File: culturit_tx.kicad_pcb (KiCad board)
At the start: 4 copper layers, 50 x 52 mm, 132 parts, among them J1 USB4105-GF-A, J2 Battery, J3 FTR-105-02-L-D, SW1 PCM12SMTR, SW2 EVQ-P7J01P, SW3 EVQ-P7J01P, U1 MCP73832T-2ACI_MC, U10 TPS22916CNYFPT, U11 SN74AUP2G08RSER, U12 TPS22916CNYFPT, U13 MDBT50Q-1M, U14 BMM150, U15 BHI260AP, U16 DS28E05R+T, U17 W25Q32JWZPIQ, U2 CSD25304W1015, U3 DMN65D8L-7, U4 CSD25304W1015, U5 TPS3839A09DBZR, U6 TPS22916CNYFPT, U7 LP5907QMFX-2.8Q1, U8 TPS6282618DMQR, U9 SN74AUP2G08RSER, Y1 32.768kHz

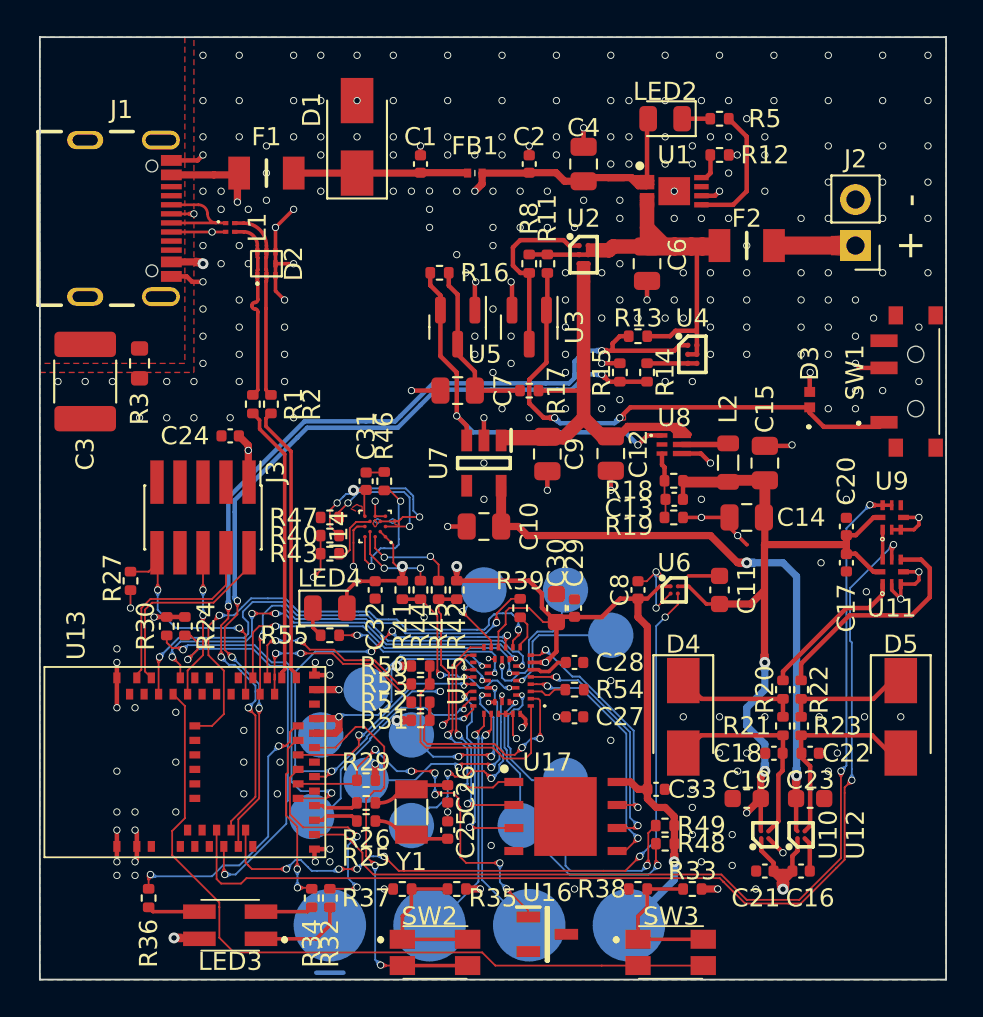
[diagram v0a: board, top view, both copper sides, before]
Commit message: 2022-08-24
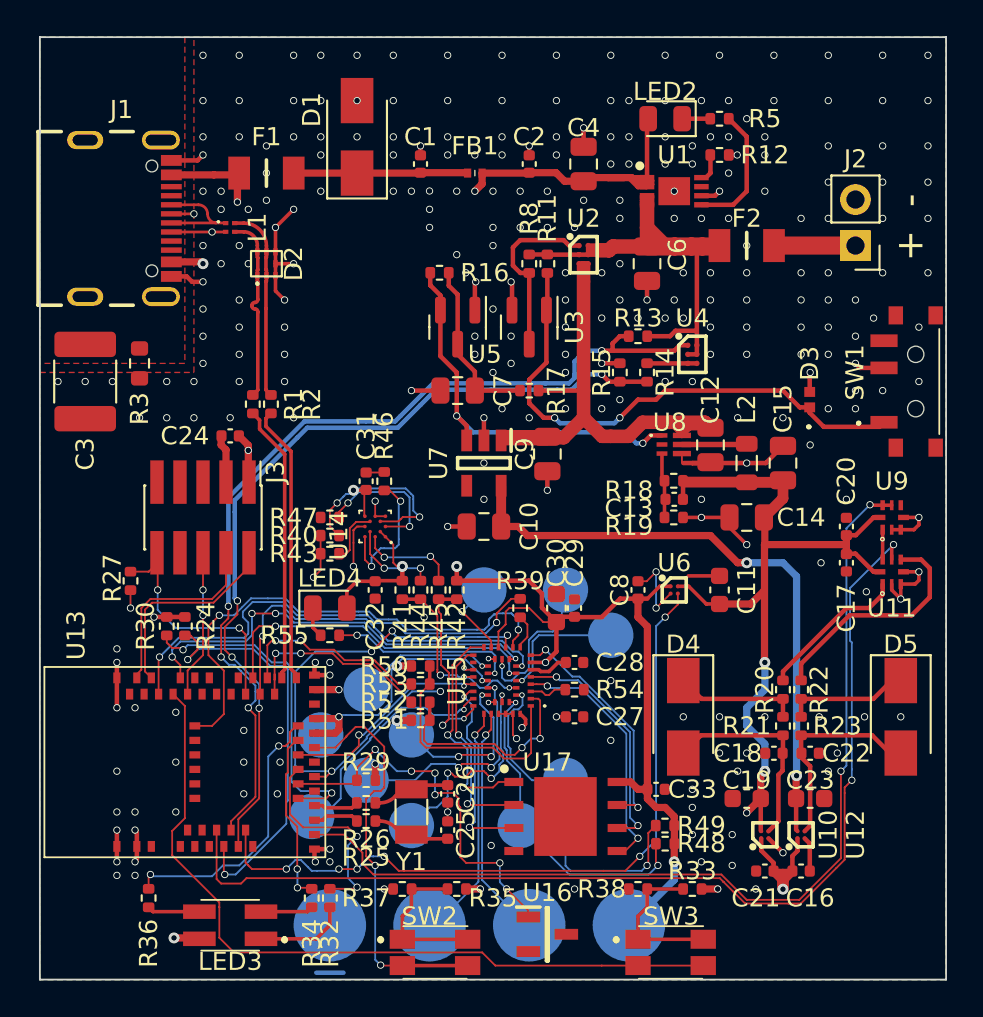
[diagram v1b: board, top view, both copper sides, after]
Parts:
- moved C12 5.52 mm to (57.0, 37.5)
- moved L2 1.03 mm to (59.0, 38.5)
- moved C15 1.00 mm to (61.0, 38.5)
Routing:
- net Earth: track 73.9 -> 79.7 mm, vias 280 -> 281
- net Net-(L2-Pad1): track 7.55 -> 3.10 mm
- net /Power/VDRAIN: track 43.7 -> 41.6 mm
- net +1V8: track 114.2 -> 115.7 mm
- net Net-(D3-Pad1): track 28.7 -> 29.5 mm

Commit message: 2022-09-07
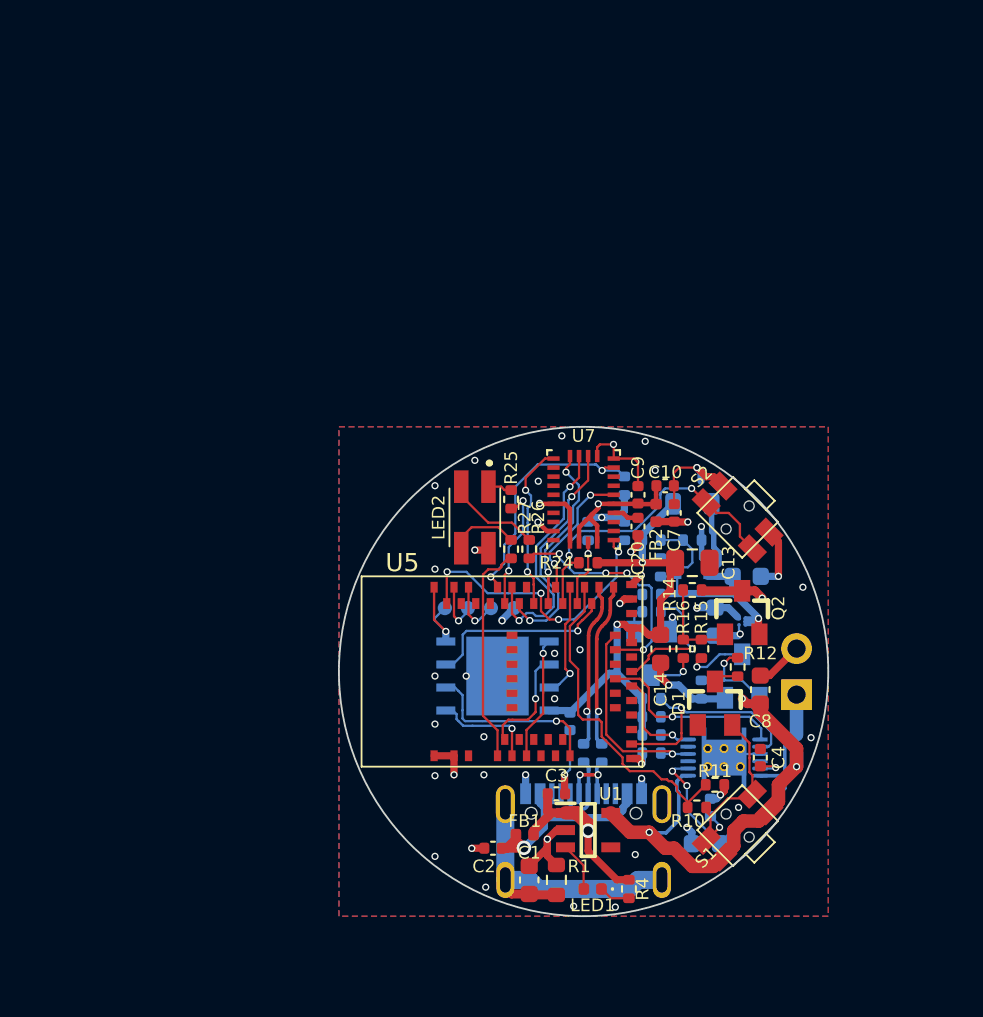
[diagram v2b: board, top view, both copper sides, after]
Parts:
- removed C15: 10uF(2012), Capacitor_SMD:C_0805_2012Metric
- removed C17, C18, C21, C22, C27, C29, C31, C32, C33: 100nF, Capacitor_SMD:C_0402_1005Metric
- removed C19, C23, C30: 1uF(1608), Capacitor_SMD:C_0603_1608Metric
- removed C24: 100pF, Capacitor_SMD:C_0402_1005Metric
- removed C25, C26: 12pF, Capacitor_SMD:C_0402_1005Metric
- removed C28: 200nF, Capacitor_SMD:C_0402_1005Metric
- removed D2: VBUS052CD-FAH-GS08, Local_devices:LLP1713-7L
- removed D3: LXES1UTAA1-157, Local_devices:LXES1UTAA1157
- removed D4, D5: SMAJ7.0A, Diode_SMD:D_SMA
- removed F1: 0ZCJ0050AF2E, Local_devices:FUSC3216X120N
- removed F2: 0ZCJ0075FF2E, Local_devices:FUSC3216X120N
- removed J3: FTR-105-02-L-D, Connector_PinHeader_1.27mm:PinHeader_2x05_P1.27mm_Vertical_SMD
- removed L2: 470nH, Inductor_SMD:L_0805_2012Metric
- removed LED3: IN-P32TATRGB, Local_devices:INP32TATRGB
- removed LED4: ORANGE, LED_SMD:LED_0805_2012Metric
- removed R22, R32: 100, Resistor_SMD:R_0402_1005Metric
- removed R23: 1.91k, Resistor_SMD:R_0402_1005Metric
- removed R33, R35: NC, Resistor_SMD:R_0402_1005Metric
- removed R34, R36: 33, Resistor_SMD:R_0402_1005Metric
- removed R37, R38: 360, Resistor_SMD:R_0402_1005Metric
- removed R39, R40, R43, R44, R45, R46, R47, R52, R53, R54: 0, Resistor_SMD:R_0402_1005Metric
- removed R41, R42, R48, R49, R50, R51: 4.7k, Resistor_SMD:R_0402_1005Metric
- removed R55: 470, Resistor_SMD:R_0402_1005Metric
- removed SW1: PCM12SMTR, Local_devices:PCM12SMTR
- removed SW2, SW3: EVQ-P7J01P, Local_devices:EVQP7J01P
- removed TP1, TP10, TP11, TP12, TP14, TP15, TP2, TP3, TP4, TP5, TP9: TestPoint, TestPoint:TestPoint_Pad_D2.5mm
- removed TP13, TP6, TP7, TP8: TestPoint, TestPoint:TestPoint_Pad_D4.0mm
- removed U10, U12: TPS22916CNYFPT, Local_devices:BGA4C40P2X2_78X78X50
- removed U11, U9: SN74AUP2G08RSER, Local_devices:RSE0008A
- removed U13: MDBT50Q-1M, Local_devices:MDBT50Q-1M
- removed U14: BMM150, Package_CSP:WLCSP-12_1.56x1.56mm_P0.4mm
- removed U15: BHI260AP, Local_devices:BHI260AP
- removed U16: DS28E05R+T, Local_devices:SOT95P237X112-3N
- removed U17: W25Q32JWZPIQ, Local_devices:SON127P600X500X80-9N-D
- removed U8: TPS6282618DMQR, Local_devices:TPS6282618DMQR
- removed Y1: 32.768kHz, Crystal:Crystal_SMD_3215-2Pin_3.2x1.5mm
- added C5: 10uF/1608, Capacitor_SMD:C_0603_1608Metric, B.Cu at (56.8, 59.5)
- added CN1: 2.54 X 2P, Connector_PinHeader_2.54mm:PinHeader_1x02_P2.54mm_Vertical, B.Cu at (61.8, 51.3)
- added FB2: MMZ1005Y121CT000, Inductor_SMD:L_0402_1005Metric, F.Cu at (54.0, 41.2)
- added LED1: APHHS1005SURCK, LED_SMD:LED_0402_1005Metric, F.Cu at (50.5, 62.0)
- added Q1: MMBT2222LT1G, Local_devices:SOT23, B.Cu at (58.8, 50.2)
- added Q2: FDN340P, Local_devices:SOT23, F.Cu at (58.8, 46.8)
- added Q3: MMBT2222LT1G, Local_devices:SOT23, B.Cu at (53.8, 49.0)
- added R10: 10k, Resistor_SMD:R_0402_1005Metric, F.Cu at (56.2, 57.5)
- added R28: 10k, Resistor_SMD:R_0402_1005Metric, B.Cu at (52.2, 39.8)
- added R4: 330, Resistor_SMD:R_0402_1005Metric, F.Cu at (52.5, 62.0)
- added R6: WFCP0402R0100FE66, Resistor_SMD:R_0402_1005Metric, B.Cu at (61.8, 54.0)
- added R7: 10k, Resistor_SMD:R_0402_1005Metric, B.Cu at (53.8, 54.5)
- added R9: 10k, Resistor_SMD:R_0402_1005Metric, B.Cu at (53.8, 51.5)
- added S1: SKSCLDE010, Local_devices:SKSCLDE010, F.Cu at (58.5, 58.5)
- added S2: SKSCLDE010, Local_devices:SKSCLDE010, F.Cu at (58.5, 41.5)
- C1: value 100nF, 16V -> 4.7nF/1608; footprint Capacitor_SMD:C_0402_1005Metric -> Capacitor_SMD:C_0603_1608Metric
- C10, C7: value 2.2uF(2012) -> 10nF; footprint Capacitor_SMD:C_0805_2012Metric -> Capacitor_SMD:C_0402_1005Metric
- C11: value 1uF(1608) -> 4.7uF/1608; moved to B.Cu
- C12: value 4.7uF(2012) -> 1uF(1608); footprint Capacitor_SMD:C_0805_2012Metric -> Capacitor_SMD:C_0603_1608Metric; moved to B.Cu
- C13: value 120pF -> 22uF/2012; footprint Capacitor_SMD:C_0402_1005Metric -> Capacitor_SMD:C_0805_2012Metric
- C14: value 10uF(2012) -> 10uF; footprint Capacitor_SMD:C_0805_2012Metric -> Capacitor_SMD:C_0603_1608Metric
- C16, R2: moved to B.Cu
- C2: value 220nF, 16V -> 10nF
- C3: value 1nF(1812),X7R,2kV -> 100nF; footprint Capacitor_SMD:C_1812_4532Metric -> Capacitor_SMD:C_0402_1005Metric
- C4: value 4.7uF(2012) -> 100nF; footprint Capacitor_SMD:C_0805_2012Metric -> Capacitor_SMD:C_0402_1005Metric
- C6: value 4.7uF(2012) -> 10nF; footprint Capacitor_SMD:C_0805_2012Metric -> Capacitor_SMD:C_0402_1005Metric; moved to B.Cu
- C8: value 100nF -> 1uF(1608); footprint Capacitor_SMD:C_0402_1005Metric -> Capacitor_SMD:C_0603_1608Metric
- C9: value 2.2uF(2012) -> 100nF; footprint Capacitor_SMD:C_0805_2012Metric -> Capacitor_SMD:C_0402_1005Metric
- D1: value SMAJ7.0A -> MMBD4148; footprint Diode_SMD:D_SMA -> Local_devices:SOT23
- FB1: value BLM15AG700SN1D -> MMZ1005Y121CT000; footprint Local_devices:BLM15AG700SN1D -> Inductor_SMD:L_0402_1005Metric
- J1: value USB4105-GF-A -> SWD; footprint Local_devices:GCT_USB4105-GF-A -> Local_devices:SWD_port; moved to B.Cu
- J2: value Battery -> USB4105-GF-A; footprint Connector_PinHeader_2.54mm:PinHeader_1x02_P2.54mm_Vertical -> Local_devices:GCT_USB4105-GF-A; moved to B.Cu
- L1: value DLM0QSN500HY2D -> 1uH/2012; footprint Local_devices:DLM0QSB120HY2D -> Inductor_SMD:L_0805_2012Metric; moved to B.Cu
- LED2: value ORANGE -> IN-P32TATRGB; footprint LED_SMD:LED_0805_2012Metric -> Local_devices:INP32TATRGB
- R1: value 22 -> 1M(1608); footprint Resistor_SMD:R_0402_1005Metric -> Resistor_SMD:R_0603_1608Metric
- R11: value 2M -> 20k
- R13: value 1M -> 20k; moved to B.Cu
- R14: value 300k -> 100k
- R15: value 180k -> 1k
- R16: value 0 -> 1k
- R17: value 1k -> 100k; moved to B.Cu
- R18: value 200k -> 1k; moved to B.Cu
- R19: value 100k -> 499k; moved to B.Cu
- R20: value 100 -> 200k; moved to B.Cu
- R21: value 1.91k -> 100k; moved to B.Cu
- R24: value 4.7k -> 10k
- R25: value 0 -> 100
- R26: value 0 -> 33
- R27: value 10k -> 33
- R29, R30: value 4.7k -> 10k; moved to B.Cu
- R3: value 1M(1608) -> 22; footprint Resistor_SMD:R_0603_1608Metric -> Resistor_SMD:R_0402_1005Metric; moved to B.Cu
- R5: value 470 -> 10k; moved to B.Cu
- R8: value 1M -> 10k; moved to B.Cu
- U1: value MCP73832T-2ACI_MC -> MAX1555EZK+T; footprint Local_devices:SON50P300X200X100-9N-D -> Local_devices:SOT95P275X110-5N
- U2: value CSD25304W1015 -> BQ27441DRZR-G1A; footprint Local_devices:BGA6C50P2X3_95X145X62 -> Local_devices:IC_BQ27441DRZR-G1A; moved to B.Cu
- U3: value DMN65D8L-7 -> TPS62A01ADRLR; footprint Package_TO_SOT_SMD:SOT-23 -> Local_devices:SOTFL50P160X60-6N; moved to B.Cu
- U4: value CSD25304W1015 -> TCR3UG33A,LF; footprint Local_devices:BGA6C50P2X3_95X145X62 -> Local_devices:BGA4N35P2X2_64X64X33; moved to B.Cu
- U5: value TPS3839A09DBZR -> MDBT50Q-1M; footprint Package_TO_SOT_SMD:SOT-23 -> Local_devices:MDBT50Q-1M
- U6: value TPS22916CNYFPT -> W25Q32JWZPIQ; footprint Local_devices:BGA4C40P2X2_78X78X50 -> Local_devices:SON127P600X500X80-9N-D; moved to B.Cu
- U7: value LP5907QMFX-2.8Q1 -> BNO055; footprint Local_devices:SOT95P280X145-5N -> Package_LGA:LGA-28_5.2x3.8mm_P0.5mm
- moved C1 40.0 mm to (47.0, 61.5)
- moved J2 38.1 mm to (50.0, 61.5)
- moved C2 37.8 mm to (45.0, 59.8), turned to 180 degrees
- moved D1 37.0 mm to (57.2, 51.8), turned to 0 degrees
- moved FB1 36.6 mm to (46.8, 59.0), turned to 180 degrees
- moved U1 35.6 mm to (50.2, 58.8)
- moved C3 34.5 mm to (48.5, 56.8), turned to 0 degrees
- moved R5 34.2 mm to (53.8, 53.5), turned to 180 degrees
- moved C4 34.2 mm to (59.8, 54.8), turned to -90 degrees
- moved R3 33.4 mm to (51.0, 54.5), turned to 90 degrees
- moved J1 32.0 mm to (46.2, 46.5), turned to 180 degrees
- moved R1 31.1 mm to (48.5, 61.5), turned to 90 degrees
- moved C6 30.2 mm to (57.0, 57.5), turned to 90 degrees
- moved R11 30.2 mm to (57.2, 56.2), turned to 0 degrees
- moved L1 29.7 mm to (56.0, 40.8), turned to 180 degrees
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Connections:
- C1 pad 1: Net-(C1-Pad1) -> GNDPWR
- C10 pad 1: Earth -> VDD_BNO
- C10 pad 2: +2V8 -> Earth
- C11 pad 1: +1V8 -> Net-(C11-Pad1)
- C12 pad 1: Earth -> +3V3
- C12 pad 2: /Power/VDRAIN -> Earth
- C13 pad 1: Net-(R18-Pad2) -> +1V8
- C13 pad 2: +1V8 -> Earth
- C14 pad 1: Earth -> +1V8
- C14 pad 2: +1V8 -> Earth
- C16 pad 1: VDD -> +1V8
- C2 pad 1: VUSB -> Net-(C2-Pad1)
- C20 pad 1: Earth -> Net-(C20-Pad1)
- C20 pad 2: +1V8 -> Earth
- C3 pad 1: GNDPWR -> VBUS
- C4 pad 1: VUSB -> Earth
- C4 pad 2: Earth -> Net-(C4-Pad2)
- C6 pad 1: +BATT -> Net-(C6-Pad1)
- C7 pad 1: Earth -> +3V3
- C7 pad 2: Net-(C7-Pad2) -> Earth
- C8 pad 1: VDDIO -> VSYS
- C9 pad 1: Earth -> VDD_BNO
- C9 pad 2: /Power/VDRAIN -> Earth
- D1 pad 1: Net-(C1-Pad1) -> unconnected-(D1-Pad1)
- D1 pad 2: Earth -> Net-(C6-Pad1)
- FB1 pad 1: Net-(C1-Pad1) -> VBUS
- FB1 pad 2: VUSB -> Net-(C2-Pad1)
- L1 pad 1: /USB Connector/DN -> Net-(L1-Pad1)
- L1 pad 2: /USB Connector/D- -> +1V8
- LED2 pad 2: VUSB -> +3V3
- R1 pad 1: /USB Connector/D+ -> GNDPWR
- R1 pad 2: /MDBT50Q/USBdata_P -> Earth
- R11 pad 1: Net-(D3-Pad1) -> /MDBT50Q/ON_MONITOR
- R11 pad 2: +BATT -> Earth
- R12 pad 1: Net-(R12-Pad1) -> Net-(D1-Pad3)
- R12 pad 2: Earth -> Net-(Q1-Pad1)
- R13 pad 1: /MDBT50Q/VBAT_MOT_EN -> Net-(Q1-Pad1)
- R13 pad 2: +BATT -> Earth
- R14 pad 1: Net-(R14-Pad1) -> VSYS
- R14 pad 2: /MDBT50Q/VBAT_MON -> Net-(Q2-Pad1)
- R15 pad 1: /MDBT50Q/VBAT_MON -> Net-(Q1-Pad3)
- R15 pad 2: Earth -> Net-(Q2-Pad1)
- R16 pad 1: Net-(C7-Pad2) -> Net-(Q3-Pad3)
- R16 pad 2: /Power/UVL_RST -> Net-(Q2-Pad1)
- R17 pad 1: /Power/VDRAIN -> Net-(C11-Pad1)
- R17 pad 2: Net-(C7-Pad2) -> Net-(Q3-Pad1)
- R18 pad 1: +1V8 -> /MDBT50Q/LDO_ON
- R18 pad 2: Net-(R18-Pad2) -> Net-(Q3-Pad1)
- R19 pad 1: Net-(R18-Pad2) -> Net-(C11-Pad1)
- R19 pad 2: Earth -> Net-(R19-Pad2)
- R2 pad 1: /USB Connector/D- -> /USB Connector/DP
- R2 pad 2: /MDBT50Q/USBdata_N -> /MDBT50Q/USBdata_P
- R20 pad 1: Net-(D4-Pad1) -> Net-(R20-Pad1)
- R20 pad 2: Net-(R20-Pad2) -> +1V8
- R21 pad 1: Net-(C18-Pad1) -> Earth
- R21 pad 2: Net-(D4-Pad1) -> Net-(R20-Pad1)
- R24 pad 1: +1V8 -> /MDBT50Q/MCU_RESET
- R24 pad 2: /MDBT50Q/SDA0 -> +1V8
- R25 pad 1: Net-(C25-Pad2) -> Net-(LED2-Pad1)
- R25 pad 2: Net-(R25-Pad2) -> /MDBT50Q/MCU_LED_R
- R26 pad 1: Net-(C26-Pad2) -> Net-(LED2-Pad3)
- R26 pad 2: Net-(R26-Pad2) -> /MDBT50Q/MCU_LED_G
- R27 pad 1: /MDBT50Q/MCU_RESET -> Net-(LED2-Pad4)
- R27 pad 2: +1V8 -> /MDBT50Q/MCU_LED_B
- R29 pad 1: /BHI260AP/PROM_RW -> +3V3
- R29 pad 2: +1V8 -> /BNO085/BNO_BOOTN
- R3 pad 1: GNDPWR -> /USB Connector/DN
- R3 pad 2: Earth -> /MDBT50Q/USBdata_N
- R30 pad 1: /MDBT50Q/SCL0 -> +3V3
- R30 pad 2: +1V8 -> /BNO085/BNO_WAKE
- R5 pad 1: Net-(LED2-Pad1) -> /MDBT50Q/GPOUT
- R5 pad 2: Net-(R5-Pad2) -> +1V8
- R8 pad 1: Net-(R8-Pad1) -> /MDBT50Q/BATT_SDA
- R8 pad 2: +BATT -> +1V8
- U1 pad 1: VUSB -> VBUS
- U1 pad 2: VUSB -> Earth
- U1 pad 3: +BATT -> Net-(LED1-Pad2)
- U1 pad 4: +BATT -> unconnected-(U1-Pad4)
- U1 pad 5: Net-(R5-Pad2) -> VSYS
- U3 pad 1: Net-(D3-Pad1) -> Earth
- U3 pad 2: Earth -> Net-(L1-Pad1)
- U3 pad 3: Net-(R8-Pad1) -> Net-(C11-Pad1)
- U4 pad A1: /MDBT50Q/VBAT_MOT_EN -> Net-(C11-Pad1)
- U4 pad A2: +BATT -> +3V3
- U4 pad B1: +BATT -> Net-(C11-Pad1)
- U4 pad B2: +BATT -> Earth
- U5 pad 2: /Power/UVL_RST -> Earth
- U5 pad 3: Net-(C7-Pad2) -> unconnected-(U5-Pad3)
- U7 pad 1: /Power/VDRAIN -> unconnected-(U7-Pad1)
- U7 pad 3: /Power/UVL_RST -> VDD_BNO
- U7 pad 4: unconnected-(U7-Pad4) -> /BNO085/BNO_BOOTN
- U7 pad 5: +2V8 -> VDD_BNO
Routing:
- net +1V8: track 115.7 -> 28.0 mm, vias 10 -> 2
- net VDDIO: track 81.8 -> 0.00 mm, vias 9 -> 0
- net +2V8: track 79.6 -> 0.00 mm, vias 3 -> 0
- net /MDBT50Q/PS_EN1: track 58.6 -> 0.00 mm, vias 2 -> 0
- net /MDBT50Q/VDD_SEL: track 53.2 -> 0.00 mm, vias 2 -> 0
- net VUSB: track 51.6 -> 0.00 mm, vias 2 -> 0
- net /MDBT50Q/VBAT_MOT_EN: track 51.2 -> 0.00 mm, vias 4 -> 0
- net /MDBT50Q/VBAT_MON: track 46.5 -> 0.00 mm, vias 4 -> 0
- net /MDBT50Q/SWITCH2: track 42.4 -> 0.00 mm
- net /Power/VDRAIN: track 41.6 -> 0.00 mm
- net /MDBT50Q/PS_EN2: track 40.5 -> 0.00 mm, vias 6 -> 0
- net VSYS: track 0.00 -> 35.8 mm, vias 0 -> 4
- net +3V3: track 0.00 -> 32.7 mm, vias 0 -> 5
- net +BATT: track 31.0 -> 0.00 mm
- net /BHI260AP/SDI/SDA: track 29.9 -> 0.00 mm, vias 5 -> 0
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- removed copper zone on In2.Cu, net +1V8
- removed copper zone on In2.Cu, net Earth
- removed copper zone on F.Cu, net GNDPWR
- removed copper zone on In2.Cu, net VDD
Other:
- board size 50 x 52 mm -> 27 x 27 mm
- board text removed: "+"
- board text removed: "-"
